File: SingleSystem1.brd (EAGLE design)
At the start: 170 x 110 mm, 43 parts, among them U1 LMZ14203, U2 SD_CARD_SOCKET, U3 XBEE

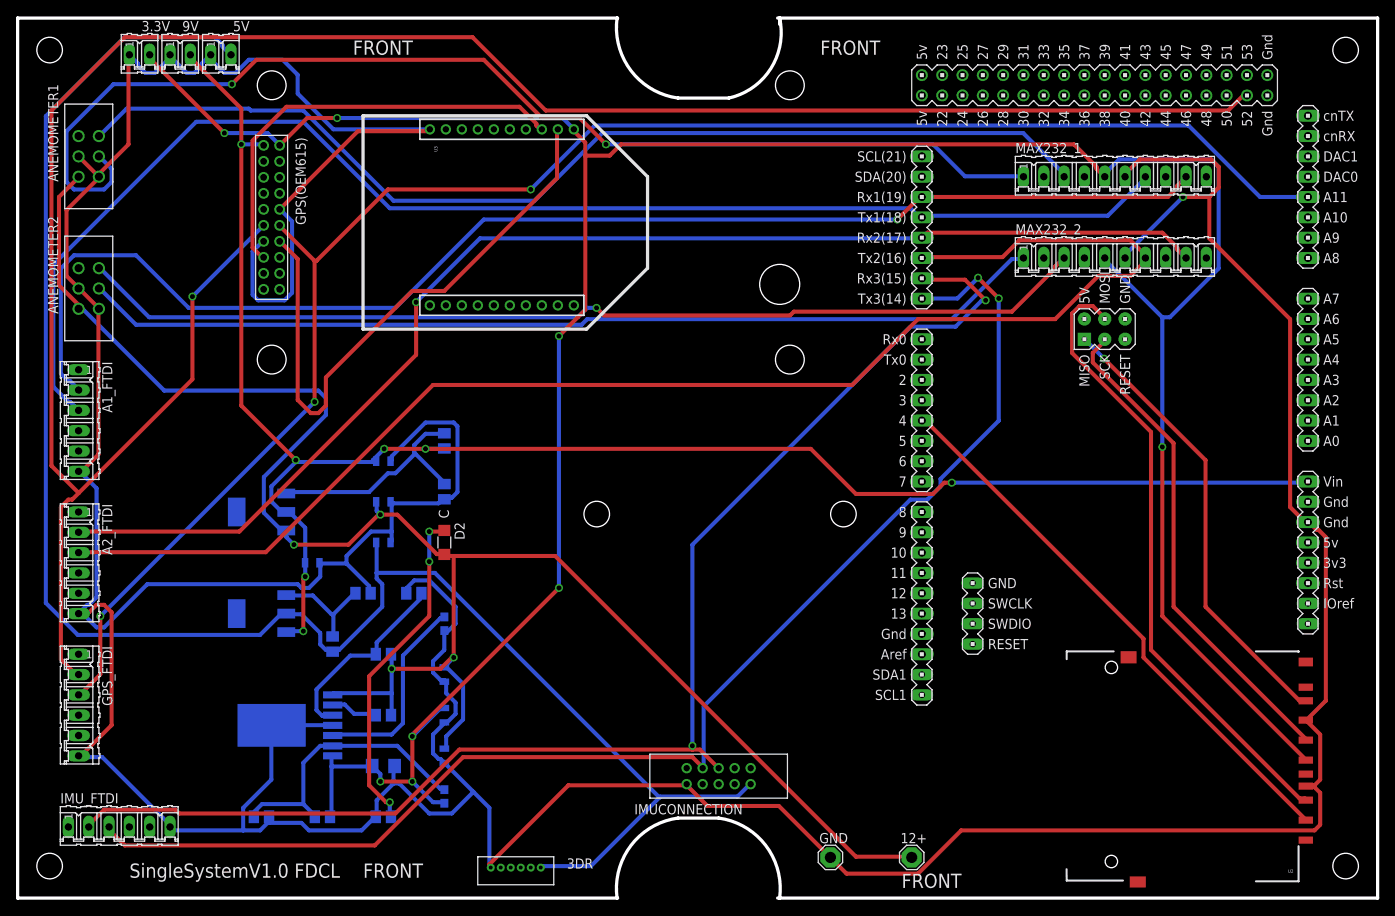
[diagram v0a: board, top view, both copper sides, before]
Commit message: edited 3DR
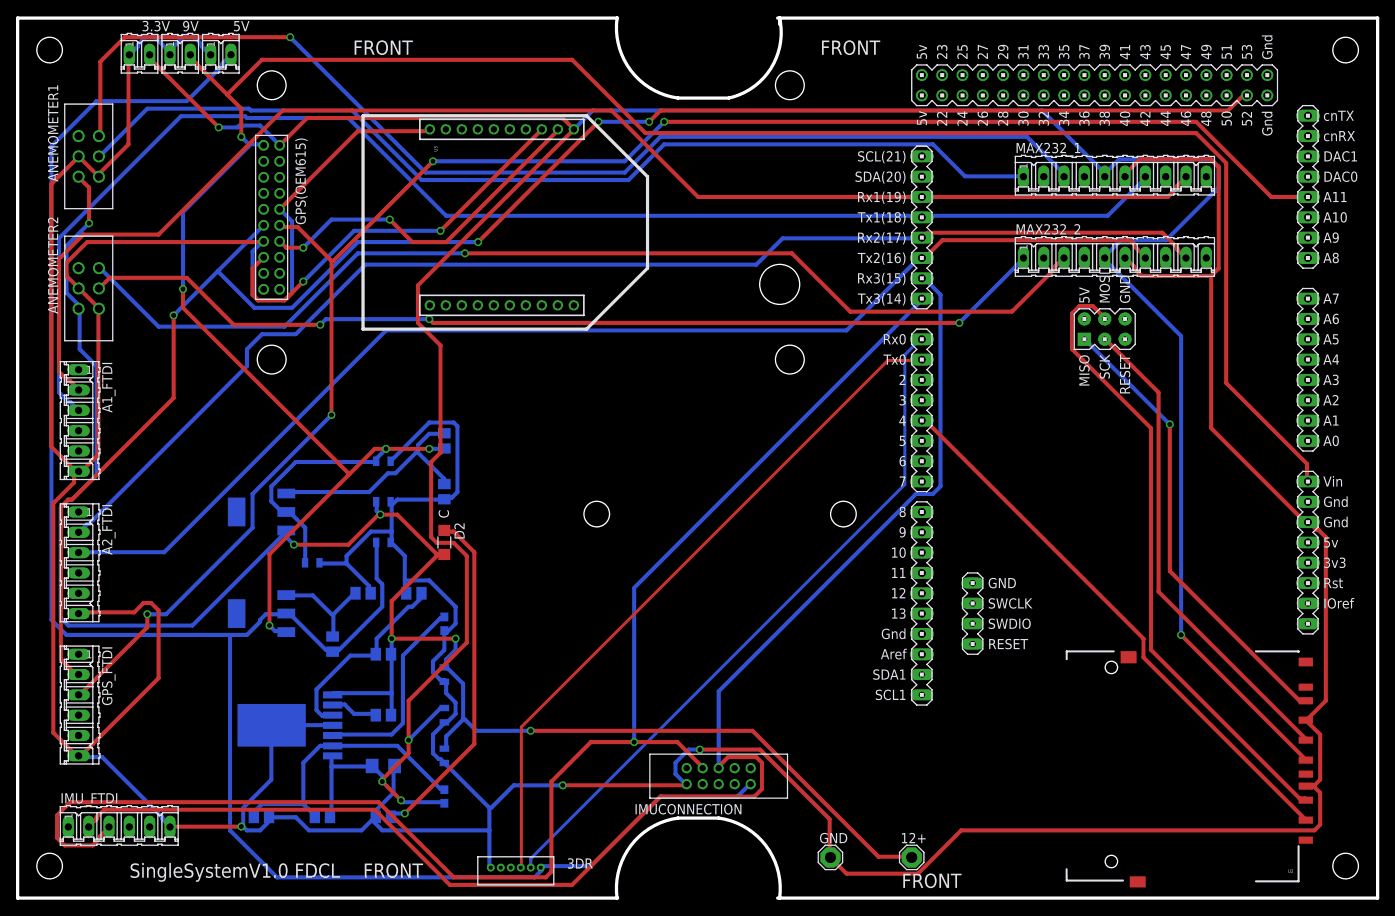
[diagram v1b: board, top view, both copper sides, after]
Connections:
- net 3DR_RX: now also U$1.TX0
- net 3DR_TX: now also U$1.RX0
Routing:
- net +9V: track 219.6 -> 312.8 mm, vias 7 -> 5
- net 3DR_RX: track 0.00 -> 86.7 mm
- net 3DR_TX: track 0.00 -> 86.6 mm
- net GPS_TX: track 275.3 -> 209.8 mm, vias 1 -> 4
- net XBEE_TX: track 74.2 -> 43.6 mm, vias 0 -> 2
- net A2_TX: track 179.0 -> 150.8 mm
- net GND: track 659.4 -> 685.0 mm, vias 1 -> 3
- net A1_IN_TX: track 146.0 -> 125.3 mm, vias 2 -> 0
- net +5V: track 225.0 -> 239.8 mm
- net IMU_RX: track 167.7 -> 181.4 mm, vias 2 -> 1
- net +12V: track 226.4 -> 238.3 mm, vias 4 -> 6
- net 3.3V: track 359.7 -> 370.1 mm, vias 8 -> 5
- net IMU_TX: track 168.5 -> 178.8 mm, vias 2 -> 0
- net A1_IN_RX: track 132.9 -> 142.3 mm, vias 0 -> 1
- net A2_IN_RX: track 127.2 -> 133.4 mm
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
